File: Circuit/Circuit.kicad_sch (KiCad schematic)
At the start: 22 parts, among them SW1 SW_DPDT_x2, SW3 SW_DPDT_x2, U1 L7805

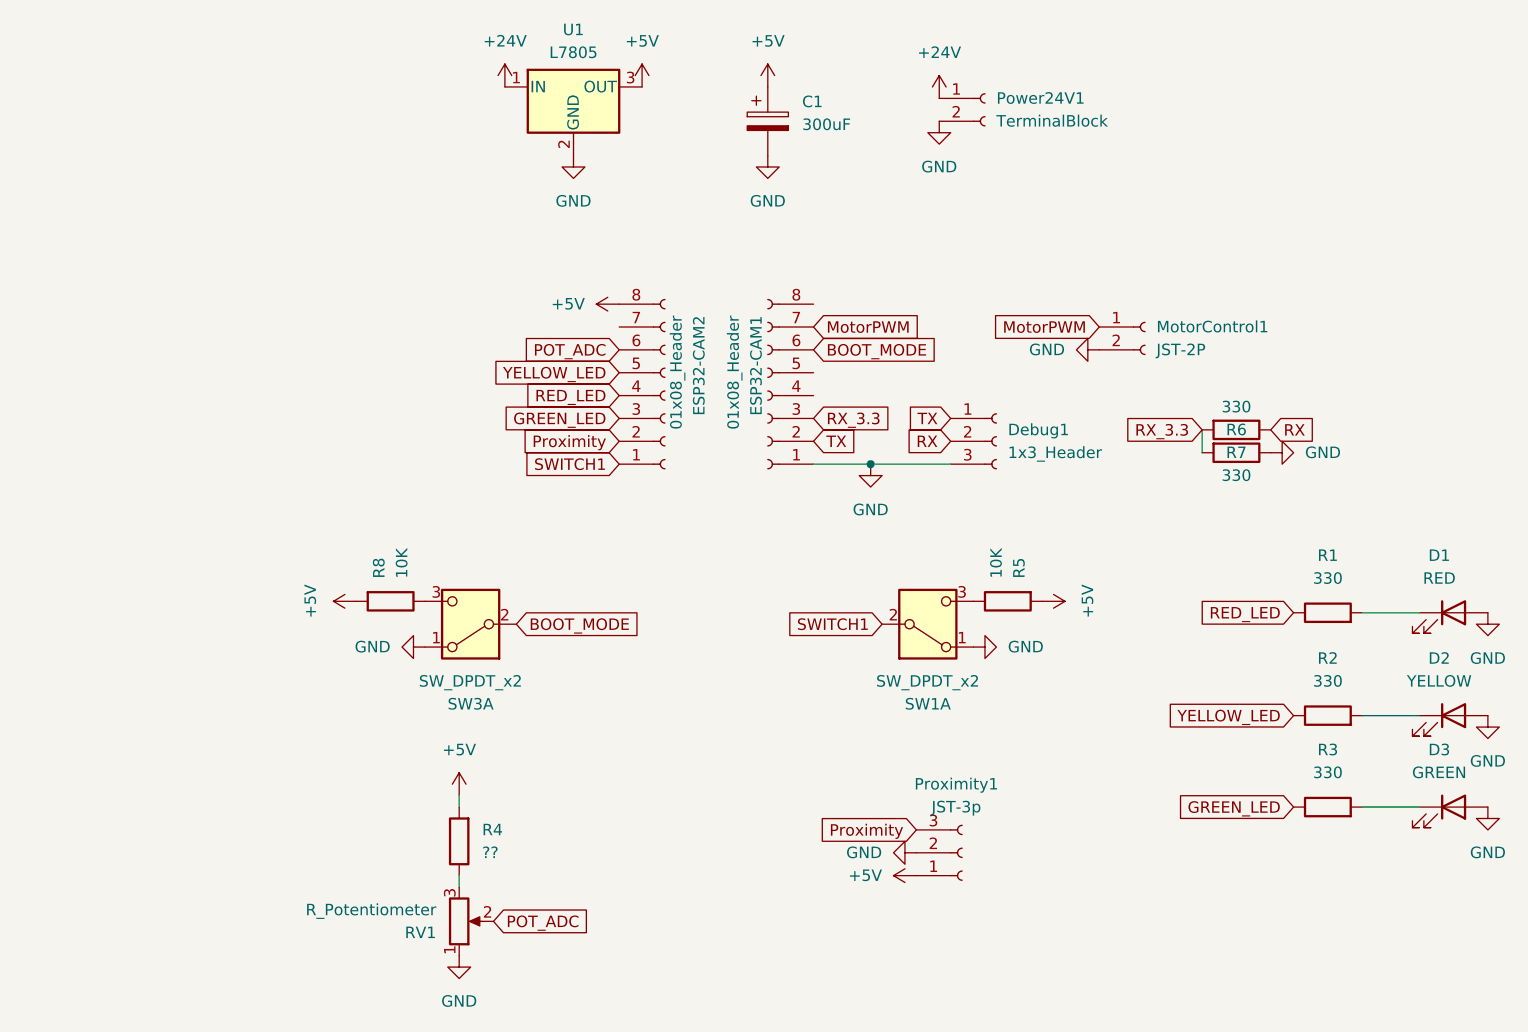
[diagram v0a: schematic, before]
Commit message: schematic and PCB modification Done
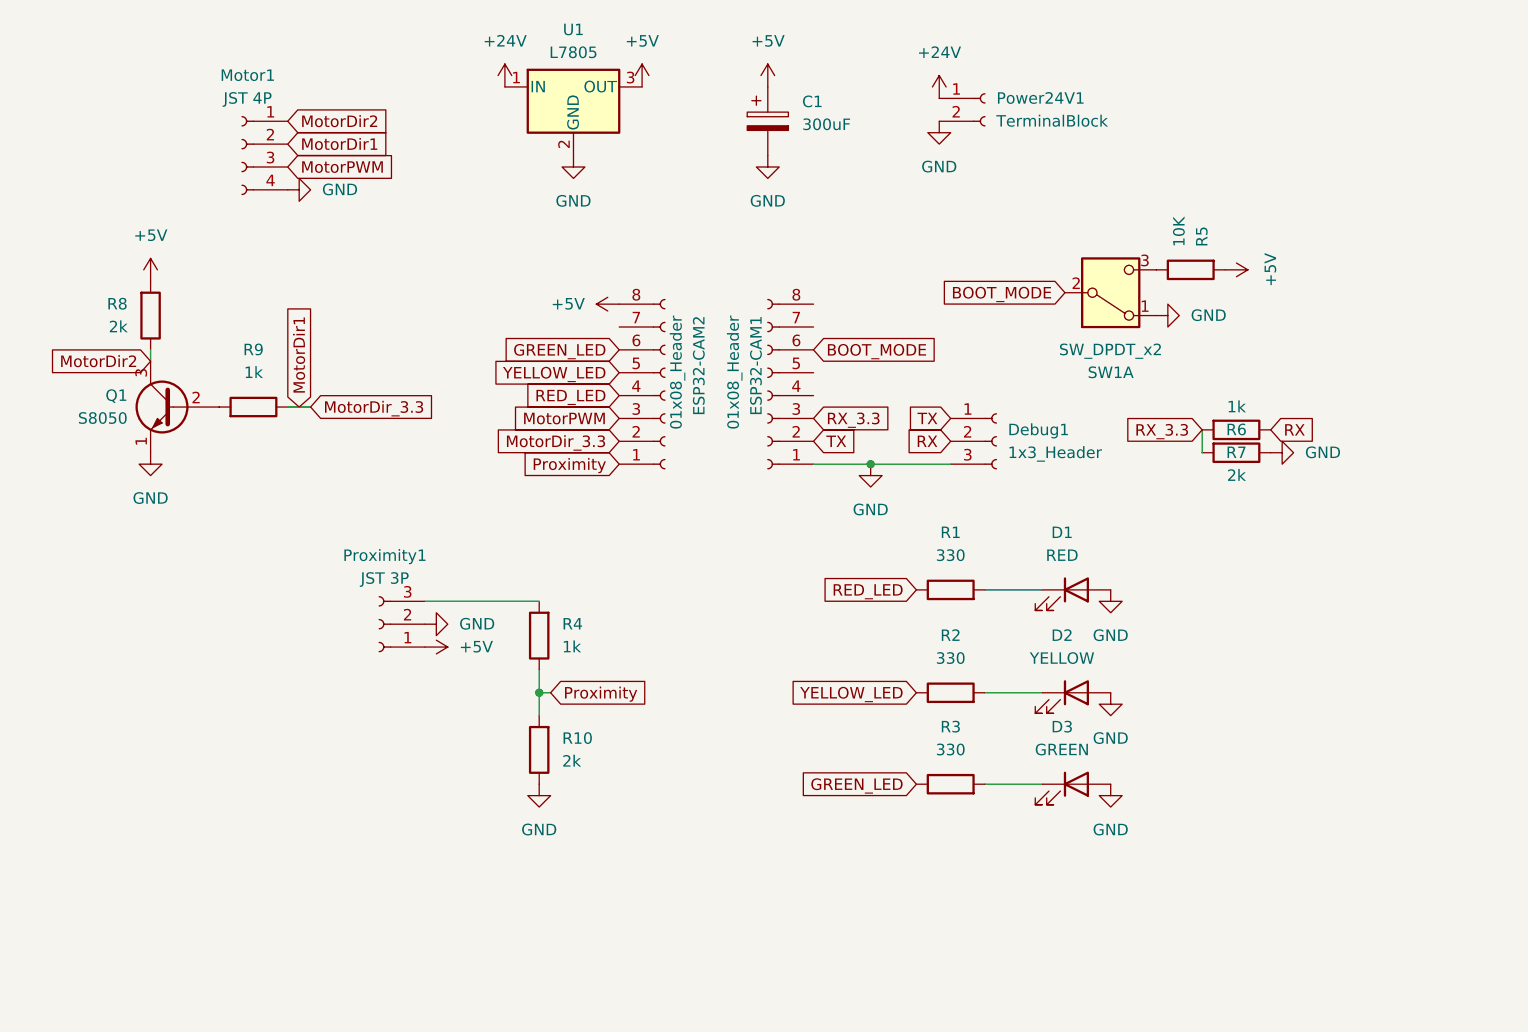
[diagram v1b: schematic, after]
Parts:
- removed MotorControl1: JST-2P, Connector_JST:JST_EH_B2B-EH-A_1x02_P2.50mm_Vertical, symbol Connector:Conn_01x02_Socket
- removed RV1: R_Potentiometer, Potentiometer_THT:Potentiometer_Alps_RK163_Single_Horizontal, symbol Device:R_Potentiometer
- removed SW3: SW_DPDT_x2, Connector_PinSocket_2.54mm:PinSocket_1x03_P2.54mm_Vertical, symbol Switch:SW_DPDT_x2
- added Motor1: JST 4P, Connector_JST:JST_EH_B4B-EH-A_1x04_P2.50mm_Vertical, symbol Connector:Conn_01x04_Socket
- added Q1: S8050, Package_TO_SOT_THT:TO-92_Inline_Wide, symbol Transistor_BJT:S8050
- added R10: 2k, Resistor_THT:R_Axial_DIN0207_L6.3mm_D2.5mm_P7.62mm_Horizontal, symbol Device:R
- added R9: 1k, Resistor_THT:R_Axial_DIN0207_L6.3mm_D2.5mm_P7.62mm_Horizontal, symbol Device:R
- Proximity1: value JST-3p -> JST 3P
- R4: value ?? -> 1k
- R6: value 330 -> 1k
- R7: value 330 -> 2k
- R8: value 10K -> 2k
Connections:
- net POT_ADC is gone; now on net GREEN_LED: ESP32-CAM2.6 (Pin_6)
- net +5V: no longer R4.2
- net BOOT_MODE: now also SW1.2 (B)
- net GND: now also Motor1.4 (Pin_4), Q1.1 (E), R10.1
- net GREEN_LED: no longer ESP32-CAM2.3 (Pin_3)
- net MotorPWM: now also ESP32-CAM2.3 (Pin_3), Motor1.3 (Pin_3); no longer ESP32-CAM1.7 (Pin_7)
- net Proximity: now also ESP32-CAM2.1 (Pin_1), R4.1, R10.2; no longer ESP32-CAM2.2 (Pin_2), Proximity1.3 (Pin_3)
- net MotorDir2: now reaches R8.1
- net MotorDir2: now also Motor1.1 (Pin_1), Q1.3 (C)
- removed net SWITCH1: ESP32-CAM2.1 (Pin_1), SW1.2 (B)
- new net: Q1.2 (B), R9.2
- new net: Proximity1.3 (Pin_3), R4.2
- new net MotorDir1: ESP32-CAM2.2 (Pin_2), Motor1.2 (Pin_2), R9.1
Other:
- moved on the sheet: D1, D2, D3, Proximity1, R1, R2, R3, R5, SW1A
